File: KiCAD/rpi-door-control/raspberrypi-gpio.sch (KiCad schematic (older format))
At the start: 21 parts, among them J1 RJ45, P1 CONN_13X2, P2 CONN_2, P3 CONN_2, P4 CONN_2, Q1 N3904, SW1 SW_PUSH, U1 RELAY

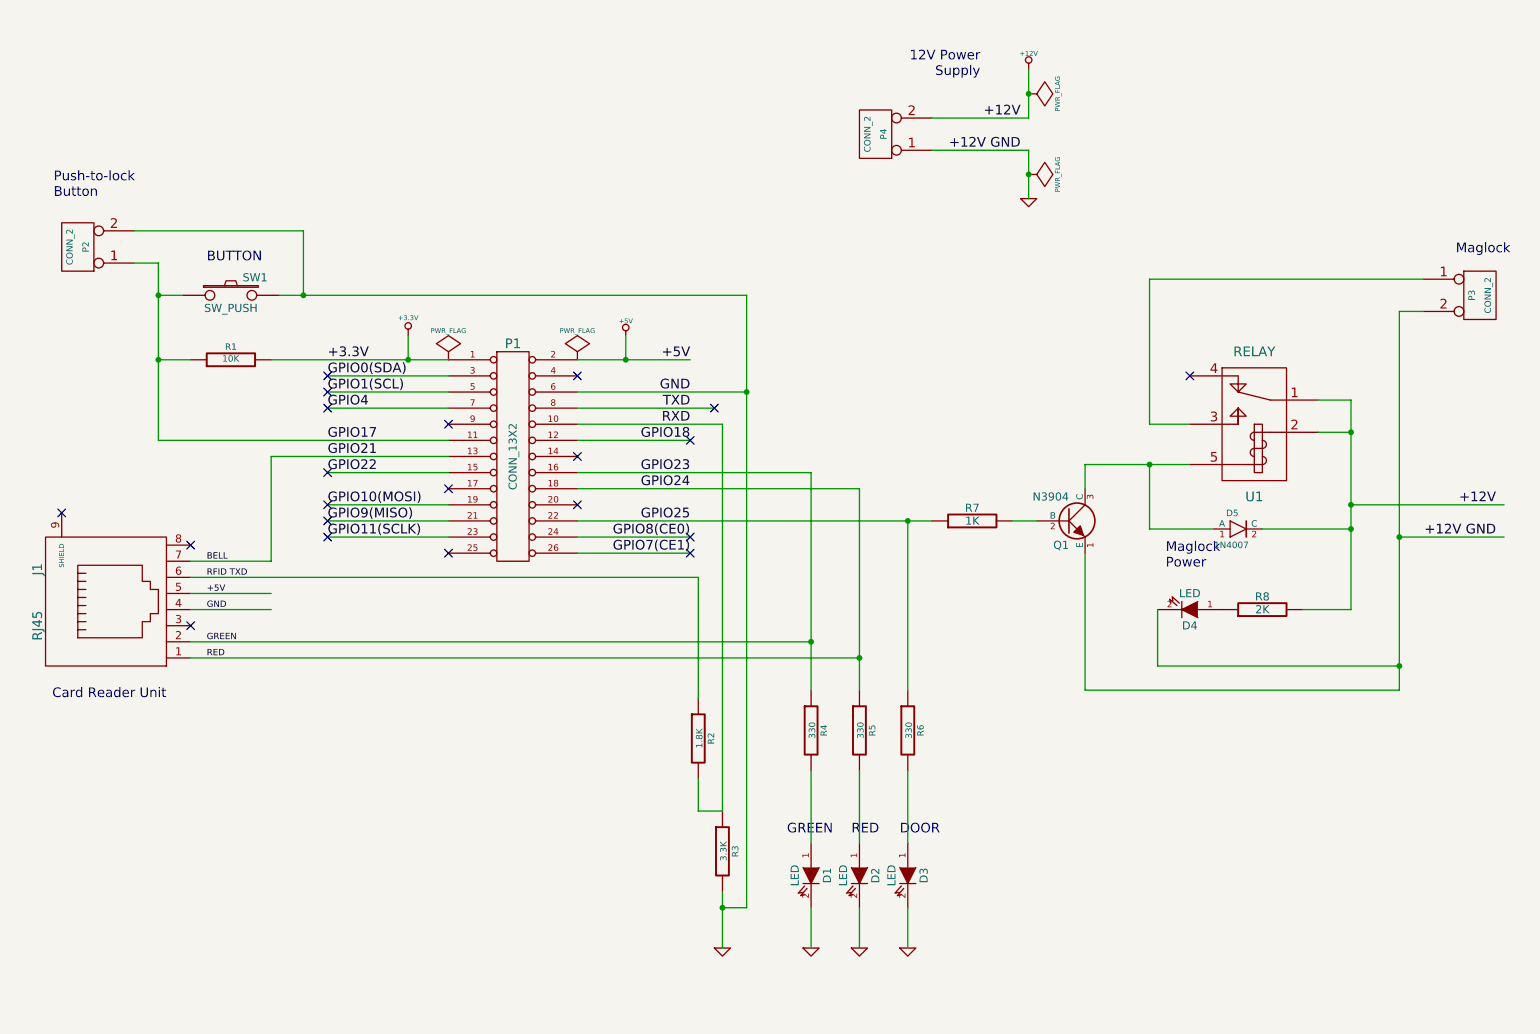
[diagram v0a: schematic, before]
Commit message: Make multi-sheet and fix stuff
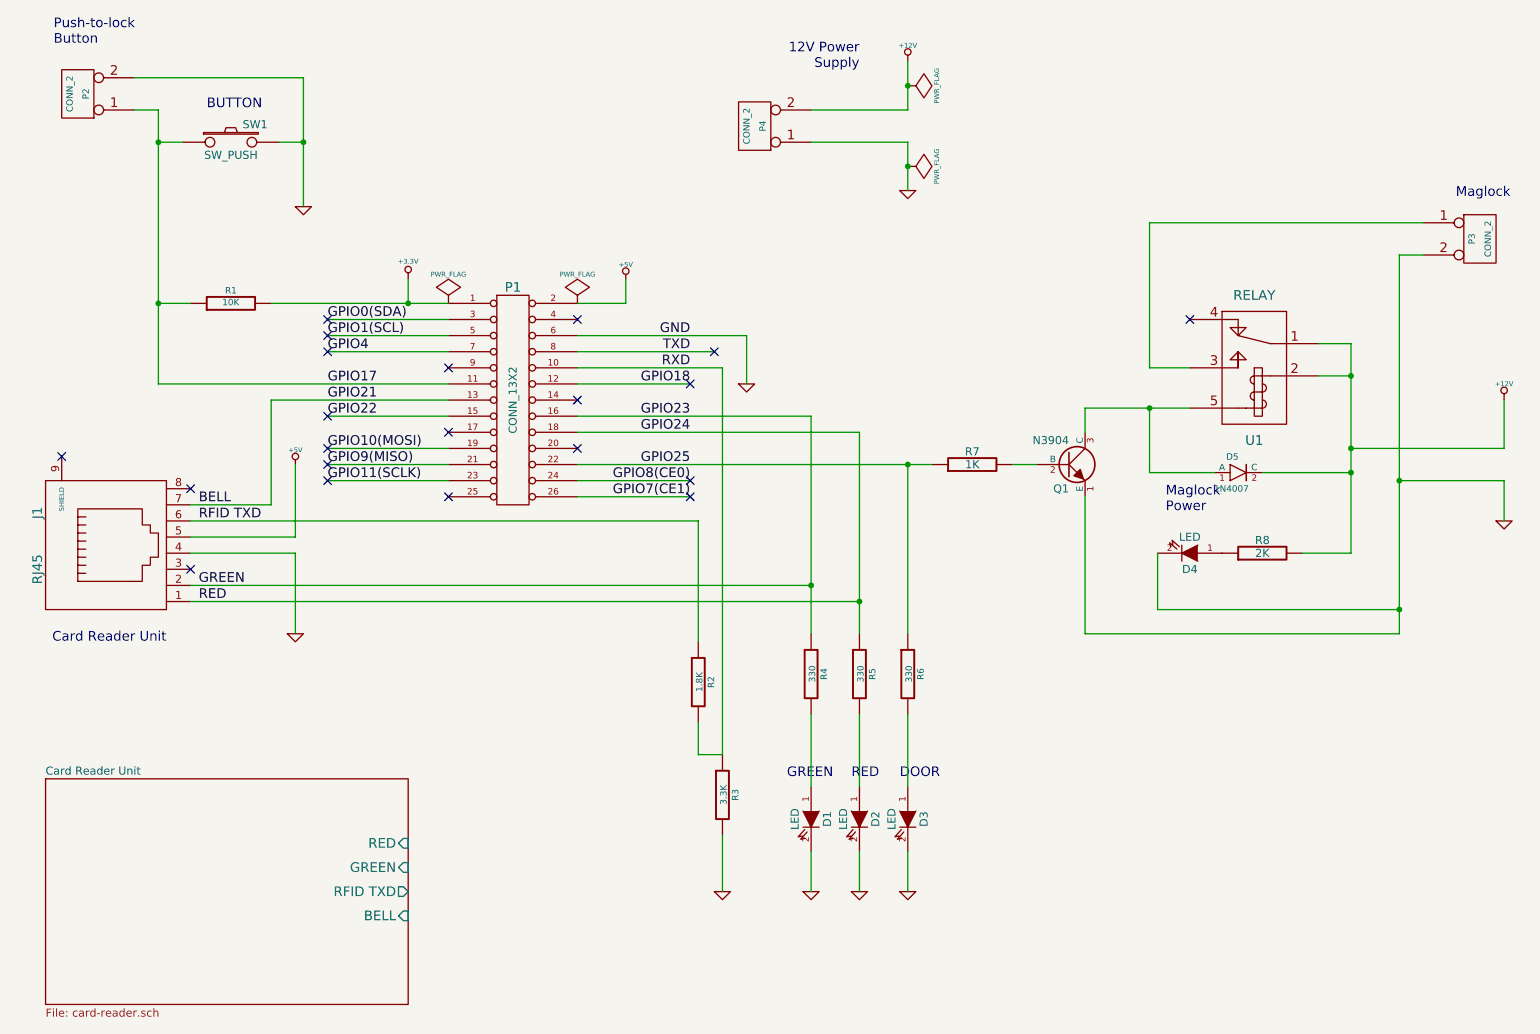
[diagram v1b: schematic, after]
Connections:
- net labels removed: +12V GND
- wire segments 77 -> 80
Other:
- moved on the sheet: D1, D2, D3, D4, D5, J1, P1, P2, P3, P4, Q1, R1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
